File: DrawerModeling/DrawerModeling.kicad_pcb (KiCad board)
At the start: 2 copper layers, 65.1 x 46.7 mm, 3 parts

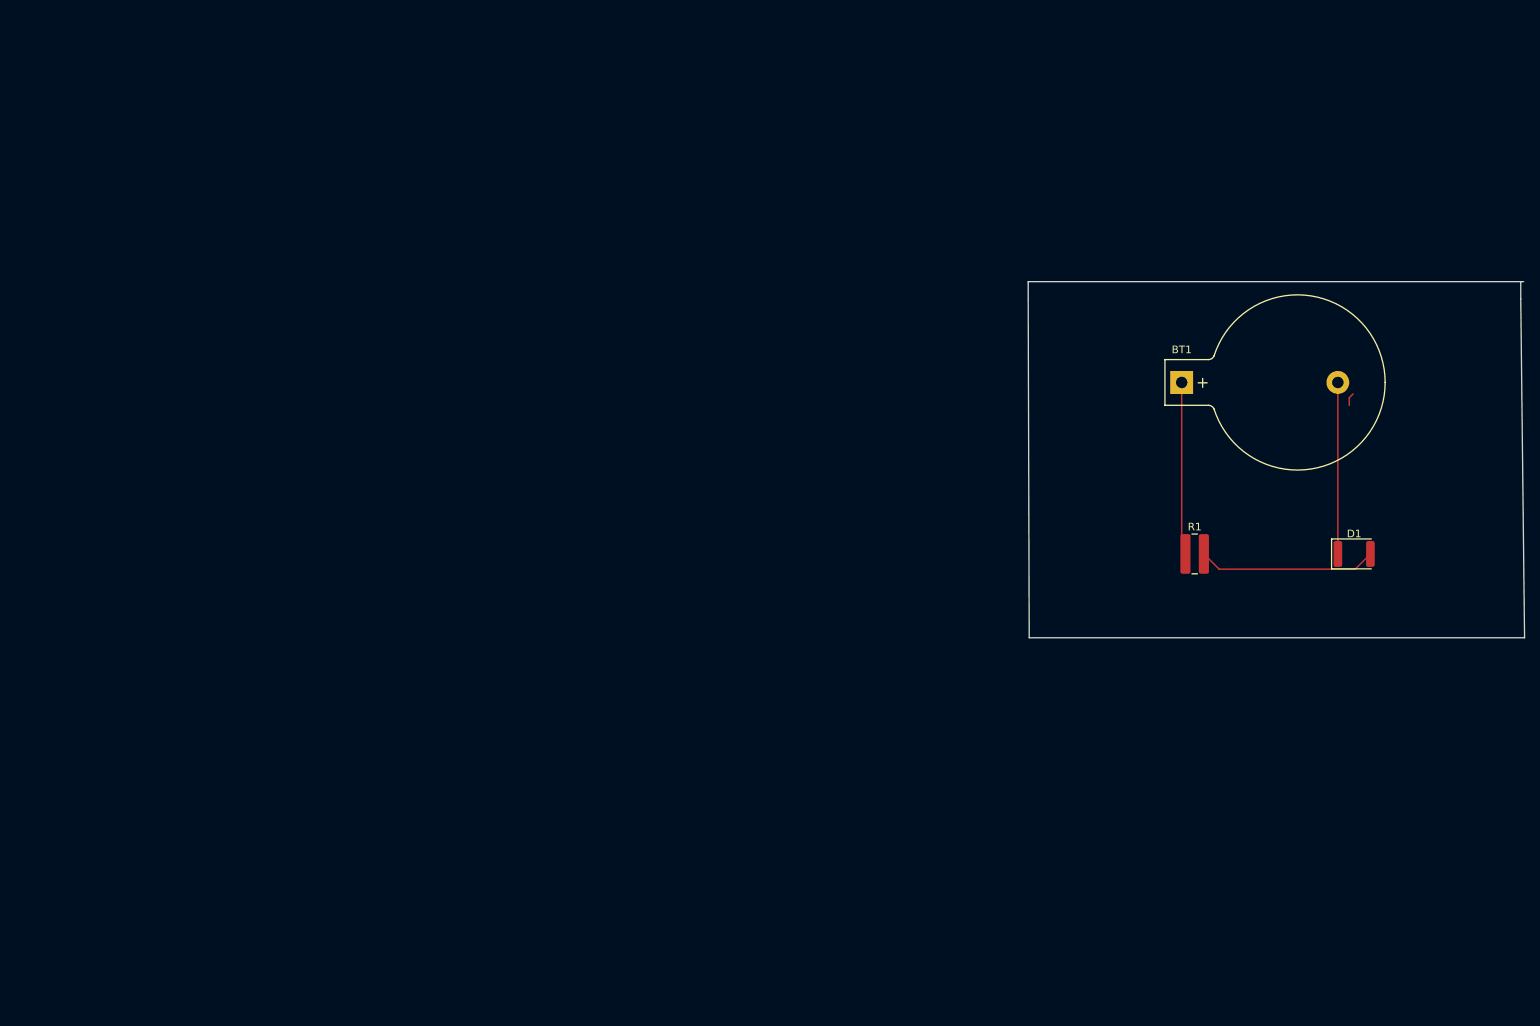
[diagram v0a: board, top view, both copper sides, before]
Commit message: pcb_1
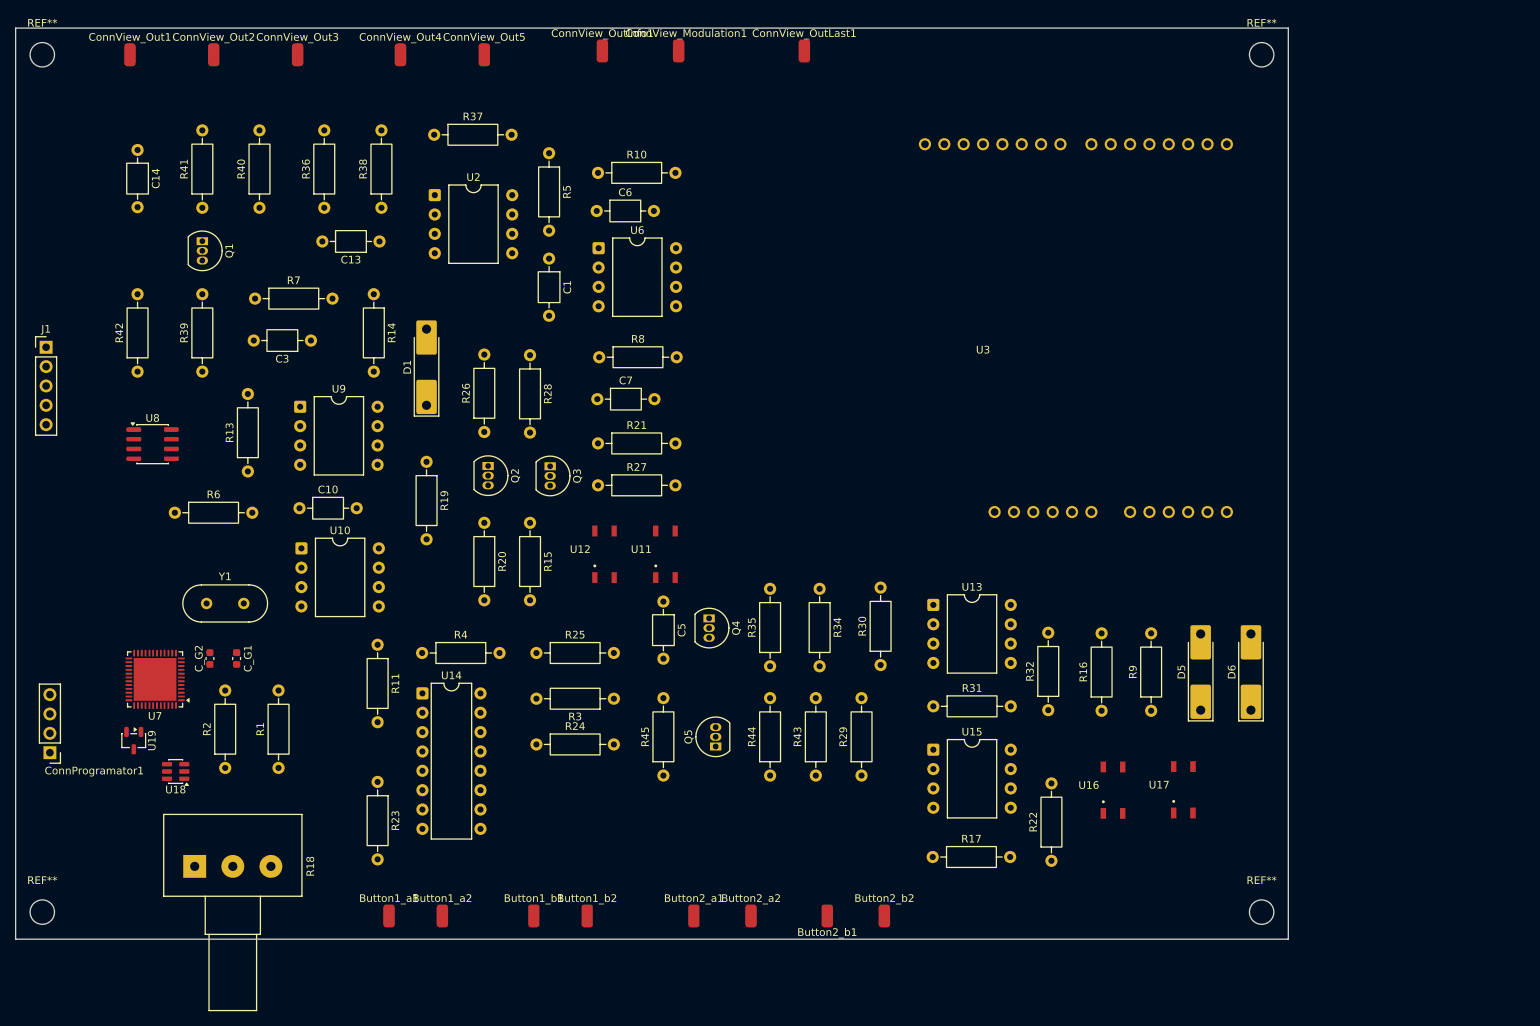
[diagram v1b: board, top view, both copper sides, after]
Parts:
- removed BT1: 9V, Battery:BatteryHolder_Keystone_103_1x20mm
- added Button1_a1: Conn_01x01, Connector_Wire:SolderWirePad_1x01_SMD_1.5x3mm, F.Cu at (70.5, 141.0)
- added Button1_a2: Conn_01x01, Connector_Wire:SolderWirePad_1x01_SMD_1.5x3mm, F.Cu at (77.5, 141.0)
- added Button1_b1: Conn_01x01, Connector_Wire:SolderWirePad_1x01_SMD_1.5x3mm, F.Cu at (89.5, 141.0)
- added Button1_b2: Conn_01x01, Connector_Wire:SolderWirePad_1x01_SMD_1.5x3mm, F.Cu at (96.5, 141.0)
- added Button2_a1: Conn_01x01, Connector_Wire:SolderWirePad_1x01_SMD_1.5x3mm, F.Cu at (110.5, 141.0)
- added Button2_a2: Conn_01x01, Connector_Wire:SolderWirePad_1x01_SMD_1.5x3mm, F.Cu at (118.0, 141.0)
- added Button2_b1: Conn_01x01, Connector_Wire:SolderWirePad_1x01_SMD_1.5x3mm, F.Cu at (128.0, 141.0)
- added Button2_b2: Conn_01x01, Connector_Wire:SolderWirePad_1x01_SMD_1.5x3mm, F.Cu at (135.5, 141.0)
- added C1: C, Capacitor_THT:C_Axial_L3.8mm_D2.6mm_P7.50mm_Horizontal, F.Cu at (91.5, 54.8)
- added C10: C, Capacitor_THT:C_Axial_L3.8mm_D2.6mm_P7.50mm_Horizontal, F.Cu at (58.8, 87.5)
- added C13: C, Capacitor_THT:C_Axial_L3.8mm_D2.6mm_P7.50mm_Horizontal, F.Cu at (69.2, 52.5)
- added C14: C, Capacitor_THT:C_Axial_L3.8mm_D2.6mm_P7.50mm_Horizontal, F.Cu at (37.5, 40.5)
- added C3: C, Capacitor_THT:C_Axial_L3.8mm_D2.6mm_P7.50mm_Horizontal, F.Cu at (60.2, 65.5)
- added C5: C, Capacitor_THT:C_Axial_L3.8mm_D2.6mm_P7.50mm_Horizontal, F.Cu at (106.5, 99.8)
- added C6: C, Capacitor_THT:C_Axial_L3.8mm_D2.6mm_P7.50mm_Horizontal, F.Cu at (97.8, 48.5)
- added C7: C, Capacitor_THT:C_Axial_L3.8mm_D2.6mm_P7.50mm_Horizontal, F.Cu at (97.8, 73.2)
- added C_G1: C, Capacitor_SMD:C_0603_1608Metric, F.Cu at (50.5, 107.2)
- added C_G2: C, Capacitor_SMD:C_0603_1608Metric, F.Cu at (47.0, 107.2)
- added ConnProgramator1: Conn_01x04_Pin, Connector_PinHeader_2.54mm:PinHeader_1x04_P2.54mm_Vertical, F.Cu at (26.0, 119.6)
- added ConnView_Modulation1: Conn_01x01, Connector_Wire:SolderWirePad_1x01_SMD_1.5x3mm, F.Cu at (108.5, 27.5)
- added ConnView_Out1: Conn_01x01, Connector_Wire:SolderWirePad_1x01_SMD_1.5x3mm, F.Cu at (36.5, 28.0)
- added ConnView_Out2: Conn_01x01, Connector_Wire:SolderWirePad_1x01_SMD_1.5x3mm, F.Cu at (47.5, 28.0)
- added ConnView_Out3: Conn_01x01, Connector_Wire:SolderWirePad_1x01_SMD_1.5x3mm, F.Cu at (58.5, 28.0)
- added ConnView_Out4: Conn_01x01, Connector_Wire:SolderWirePad_1x01_SMD_1.5x3mm, F.Cu at (72.0, 28.0)
- added ConnView_Out5: Conn_01x01, Connector_Wire:SolderWirePad_1x01_SMD_1.5x3mm, F.Cu at (83.0, 28.0)
- added ConnView_OutInfo1: Conn_01x01, Connector_Wire:SolderWirePad_1x01_SMD_1.5x3mm, F.Cu at (98.5, 27.5)
- added ConnView_OutLast1: Conn_01x01, Connector_Wire:SolderWirePad_1x01_SMD_1.5x3mm, F.Cu at (125.0, 27.5)
- added D5: D, Diode_SMD:D_MELF-RM10_Universal_Handsoldering, F.Cu at (177.0, 109.0)
- added D6: D, Diode_SMD:D_MELF-RM10_Universal_Handsoldering, F.Cu at (183.6, 109.0)
- added J1: Conn_01x05_Pin, Connector_PinHeader_2.54mm:PinHeader_1x05_P2.54mm_Vertical, F.Cu at (25.5, 66.4)
- added Q1: 2N3904, Package_TO_SOT_THT:TO-92_Inline, F.Cu at (46.0, 52.5)
- added Q2: 2N3904, Package_TO_SOT_THT:TO-92_Inline, F.Cu at (83.5, 82.0)
- added Q3: 2N3906, Package_TO_SOT_THT:TO-92_Inline, F.Cu at (91.6, 82.0)
- added Q4: 2N3904, Package_TO_SOT_THT:TO-92_Inline, F.Cu at (112.5, 102.0)
- added Q5: 2N3904, Package_TO_SOT_THT:TO-92_Inline, F.Cu at (113.4, 118.8)
- added R10: R, Resistor_THT:R_Axial_DIN0207_L6.3mm_D2.5mm_P10.16mm_Horizontal, F.Cu at (97.9, 43.5)
- added R11: R, Resistor_THT:R_Axial_DIN0207_L6.3mm_D2.5mm_P10.16mm_Horizontal, F.Cu at (69.0, 105.4)
- added R13: R, Resistor_THT:R_Axial_DIN0207_L6.3mm_D2.5mm_P10.16mm_Horizontal, F.Cu at (52.0, 82.7)
- added R14: R, Resistor_THT:R_Axial_DIN0207_L6.3mm_D2.5mm_P10.16mm_Horizontal, F.Cu at (68.5, 59.4)
- added R15: R, Resistor_THT:R_Axial_DIN0207_L6.3mm_D2.5mm_P10.16mm_Horizontal, F.Cu at (89.0, 89.4)
- added R16: R, Resistor_THT:R_Axial_DIN0207_L6.3mm_D2.5mm_P10.16mm_Horizontal, F.Cu at (164.0, 114.1)
- added R17: R, Resistor_THT:R_Axial_DIN0207_L6.3mm_D2.5mm_P10.16mm_Horizontal, F.Cu at (141.8, 133.3)
- added R18: R_Potentiometer_US, Potentiometer_THT:Potentiometer_Alps_RK163_Single_Horizontal, F.Cu at (45.0, 134.5)
- added R19: R, Resistor_THT:R_Axial_DIN0207_L6.3mm_D2.5mm_P10.16mm_Horizontal, F.Cu at (75.4, 81.4)
- added R2: 4.7k, Resistor_THT:R_Axial_DIN0207_L6.3mm_D2.5mm_P10.16mm_Horizontal, F.Cu at (49.0, 121.6)
- added R20: R, Resistor_THT:R_Axial_DIN0207_L6.3mm_D2.5mm_P10.16mm_Horizontal, F.Cu at (83.0, 89.4)
- added R21: R, Resistor_THT:R_Axial_DIN0207_L6.3mm_D2.5mm_P10.16mm_Horizontal, F.Cu at (97.9, 79.0)
- added R22: R, Resistor_THT:R_Axial_DIN0207_L6.3mm_D2.5mm_P10.16mm_Horizontal, F.Cu at (157.4, 133.8)
- added R23: R, Resistor_THT:R_Axial_DIN0207_L6.3mm_D2.5mm_P10.16mm_Horizontal, F.Cu at (69.0, 123.4)
- added R24: R, Resistor_THT:R_Axial_DIN0207_L6.3mm_D2.5mm_P10.16mm_Horizontal, F.Cu at (89.8, 118.5)
- added R25: R, Resistor_THT:R_Axial_DIN0207_L6.3mm_D2.5mm_P10.16mm_Horizontal, F.Cu at (89.8, 106.5)
- added R26: R, Resistor_THT:R_Axial_DIN0207_L6.3mm_D2.5mm_P10.16mm_Horizontal, F.Cu at (83.0, 77.5)
- added R27: R, Resistor_THT:R_Axial_DIN0207_L6.3mm_D2.5mm_P10.16mm_Horizontal, F.Cu at (97.9, 84.5)
- added R28: R, Resistor_THT:R_Axial_DIN0207_L6.3mm_D2.5mm_P10.16mm_Horizontal, F.Cu at (89.0, 67.4)
- added R29: R, Resistor_THT:R_Axial_DIN0207_L6.3mm_D2.5mm_P10.16mm_Horizontal, F.Cu at (132.5, 122.6)
- added R3: R, Resistor_THT:R_Axial_DIN0207_L6.3mm_D2.5mm_P10.16mm_Horizontal, F.Cu at (100.0, 112.5)
- added R30: R, Resistor_THT:R_Axial_DIN0207_L6.3mm_D2.5mm_P10.16mm_Horizontal, F.Cu at (135.0, 108.1)
- added R31: R, Resistor_THT:R_Axial_DIN0207_L6.3mm_D2.5mm_P10.16mm_Horizontal, F.Cu at (141.9, 113.5)
- added R32: R, Resistor_THT:R_Axial_DIN0207_L6.3mm_D2.5mm_P10.16mm_Horizontal, F.Cu at (157.0, 114.0)
- added R34: R, Resistor_THT:R_Axial_DIN0207_L6.3mm_D2.5mm_P10.16mm_Horizontal, F.Cu at (127.0, 98.1)
- added R35: R, Resistor_THT:R_Axial_DIN0207_L6.3mm_D2.5mm_P10.16mm_Horizontal, F.Cu at (120.5, 108.2)
- added R36: R, Resistor_THT:R_Axial_DIN0207_L6.3mm_D2.5mm_P10.16mm_Horizontal, F.Cu at (62.0, 48.1)
- added R37: R, Resistor_THT:R_Axial_DIN0207_L6.3mm_D2.5mm_P10.16mm_Horizontal, F.Cu at (76.4, 38.5)
- added R38: R, Resistor_THT:R_Axial_DIN0207_L6.3mm_D2.5mm_P10.16mm_Horizontal, F.Cu at (69.5, 48.1)
- added R39: R, Resistor_THT:R_Axial_DIN0207_L6.3mm_D2.5mm_P10.16mm_Horizontal, F.Cu at (46.0, 69.6)
- added R4: R, Resistor_THT:R_Axial_DIN0207_L6.3mm_D2.5mm_P10.16mm_Horizontal, F.Cu at (74.8, 106.5)
- added R40: R, Resistor_THT:R_Axial_DIN0207_L6.3mm_D2.5mm_P10.16mm_Horizontal, F.Cu at (53.5, 48.1)
- added R41: R, Resistor_THT:R_Axial_DIN0207_L6.3mm_D2.5mm_P10.16mm_Horizontal, F.Cu at (46.0, 48.1)
- added R42: R, Resistor_THT:R_Axial_DIN0207_L6.3mm_D2.5mm_P10.16mm_Horizontal, F.Cu at (37.5, 69.6)
- added R43: R, Resistor_THT:R_Axial_DIN0207_L6.3mm_D2.5mm_P10.16mm_Horizontal, F.Cu at (126.5, 122.6)
- added R44: R, Resistor_THT:R_Axial_DIN0207_L6.3mm_D2.5mm_P10.16mm_Horizontal, F.Cu at (120.5, 122.6)
- added R45: R, Resistor_THT:R_Axial_DIN0207_L6.3mm_D2.5mm_P10.16mm_Horizontal, F.Cu at (106.5, 122.6)
- added R5: R, Resistor_THT:R_Axial_DIN0207_L6.3mm_D2.5mm_P10.16mm_Horizontal, F.Cu at (91.5, 40.9)
- added R6: R, Resistor_THT:R_Axial_DIN0207_L6.3mm_D2.5mm_P10.16mm_Horizontal, F.Cu at (42.4, 88.1)
- added R7: R, Resistor_THT:R_Axial_DIN0207_L6.3mm_D2.5mm_P10.16mm_Horizontal, F.Cu at (52.9, 60.0)
- added R8: R, Resistor_THT:R_Axial_DIN0207_L6.3mm_D2.5mm_P10.16mm_Horizontal, F.Cu at (98.1, 67.7)
- added R9: R, Resistor_THT:R_Axial_DIN0207_L6.3mm_D2.5mm_P10.16mm_Horizontal, F.Cu at (170.5, 114.1)
- added REF**: MountingHole_3.2mm_M3, MountingHole:MountingHole_3.2mm_M3, F.Cu at (25.0, 140.5)
- added REF**: MountingHole_3.2mm_M3, MountingHole:MountingHole_3.2mm_M3, F.Cu at (25.0, 28.0)
- added REF**: MountingHole_3.2mm_M3, MountingHole:MountingHole_3.2mm_M3, F.Cu at (185.0, 140.5)
- added REF**: MountingHole_3.2mm_M3, MountingHole:MountingHole_3.2mm_M3, F.Cu at (185.0, 28.0)
- added U10: TL072, Package_DIP:DIP-8_W10.16mm, F.Cu at (59.0, 92.8)
- added U11: TLP222A, VikLib:TLP127, F.Cu at (106.8, 93.5)
- added U12: TLP222A, VikLib:TLP127, F.Cu at (98.8, 93.5)
- added U13: TL072, Package_DIP:DIP-8_W10.16mm, F.Cu at (141.9, 100.2)
- added U14: LM13700, Package_DIP:DIP-16_W7.62mm, F.Cu at (74.9, 111.8)
- added U15: TL072, Package_DIP:DIP-8_W10.16mm, F.Cu at (141.9, 119.2)
- added U16: TLP222A, VikLib:TLP127, F.Cu at (165.5, 124.5)
- added U17: TLP222A, VikLib:TLP127, F.Cu at (174.7, 124.5)
- added U18: MCP4725xxx-xCH, Package_TO_SOT_SMD:SOT-23-6, F.Cu at (42.5, 122.0)
- added U19: XC6206PxxxMR, Package_TO_SOT_SMD:SOT-23-3, F.Cu at (37.0, 118.0)
- added U2: TL072, Package_DIP:DIP-8_W10.16mm, F.Cu at (76.5, 46.4)
- added U3: ~, Audio_Module:Arduino_LCD_Shield, F.Cu at (148.3, 61.2)
- added U6: TL072, Package_DIP:DIP-8_W10.16mm, F.Cu at (98.0, 53.4)
- added U7: STM32F411CCUx, Package_DFN_QFN:QFN-48-1EP_7x7mm_P0.5mm_EP5.6x5.6mm, F.Cu at (39.8, 110.0)
- added U8: LT1011, Package_SO:SOIC-8_3.9x4.9mm_P1.27mm, F.Cu at (39.5, 79.1)
- added U9: TL072, Package_DIP:DIP-8_W10.16mm, F.Cu at (58.8, 74.2)
- added Y1: Crystal, Crystal:Crystal_HC49-U_Vertical, F.Cu at (46.6, 100.0)
- D1: value LED -> D; footprint LED_SMD:LED_1812_4532Metric -> Diode_SMD:D_MELF-RM10_Universal_Handsoldering
- R1: value 420 -> 4.7k; footprint Resistor_SMD:R_1020_2550Metric_Pad1.33x5.20mm_HandSolder -> Resistor_THT:R_Axial_DIN0207_L6.3mm_D2.5mm_P10.16mm_Horizontal
- moved D1 124.2 mm to (75.4, 69.0), turned to 90 degrees
- moved R1 123.4 mm to (56.0, 121.6), turned to 90 degrees
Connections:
- R1 pad 1: Net-(BT1-+) -> /V5
- R1 pad 2: Net-(D1-A) -> /SCL
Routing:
- net Net-(D1-A): track 23.5 -> 0.00 mm
- net Net-(BT1-+): track 22.7 -> 0.00 mm
- net Net-(Button1_a1-Pin_1): track 22.5 -> 0.00 mm
- net (no net): track 1.71 -> 0.00 mm
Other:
- board size 65.1 x 46.7 mm -> 167 x 119.6 mm
